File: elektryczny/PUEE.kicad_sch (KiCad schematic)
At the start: 61 parts, among them J1 CAN, J2 VIN, J4 Button1, J5 LED1, J6 Button2, J7 STM, J8 OLED, SW1 Button2, SW2 Button1, U1 STM32F042F4Px, U10 WS2815, U11 WS2815, U13 SN65HVD230QDRG4Q1, U2 ESP-12E, U3 TPS54308, U4 WS2815, U5 WS2815, U6 WS2815, U7 WS2815, U8 WS2815, U9 WS2815, Y2 ABL-8MHZ-B2

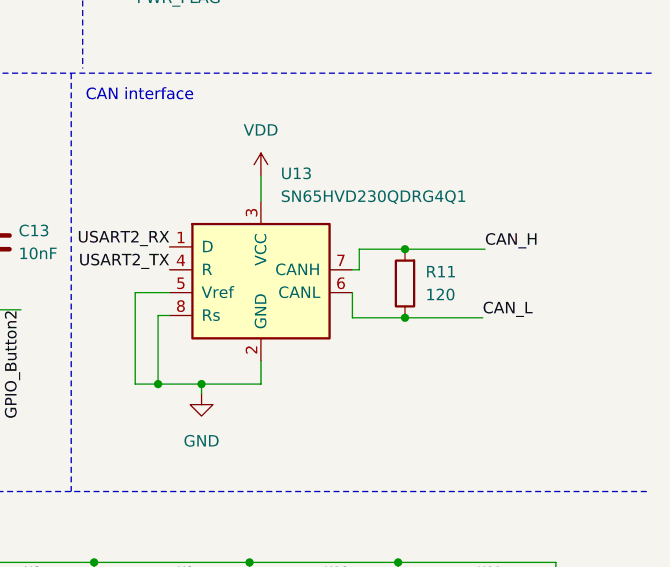
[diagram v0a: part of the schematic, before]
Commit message: polaczenia attempt 1, do poprawki
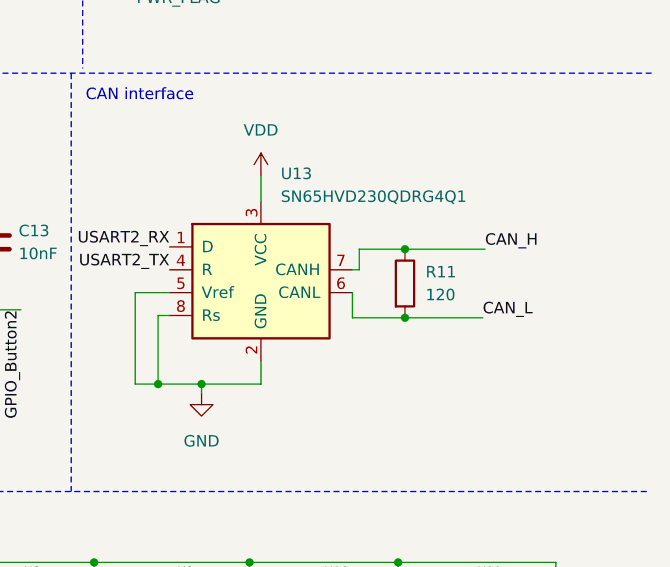
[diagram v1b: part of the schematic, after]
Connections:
- net CAN_H: now also R11.1; no longer R11.2
- net CAN_L: now also R11.2; no longer R11.1
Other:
- moved on the sheet: R11
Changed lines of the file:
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@@
 	)
 	(junction
-		(at 258.064 109.728)
+		(at 240.792 144.526)
 		(diameter 0)
 		(color 0 0 0 0)
 	)
 	(junction
-		(at 240.792 144.526)
+		(at 20.828 122.174)
 		(diameter 0)
 		(color 0 0 0 0)
 	)
 	(junction
-		(at 20.828 122.174)
+		(at 258.064 117.348)
 		(diameter 0)
 		(color 0 0 0 0)
@@
 	)
 	(junction
-		(at 258.064 117.348)
+		(at 258.064 109.728)
 		(diameter 0)
 		(color 0 0 0 0)
@@
 	(wire
 		(pts
-			(xy 258.064 117.348) (xy 266.7 117.348)
-		)
-		(stroke
-			(width 0)
-			(type default)
-		)
-	)
-	(wire
-		(pts
 			(xy 183.896 116.078) (xy 186.436 116.078)
 		)
@@
 	(wire
 		(pts
-			(xy 258.064 109.728) (xy 266.954 109.728)
+			(xy 206.756 162.052) (xy 206.756 163.322)
 		)
 		(stroke
@@
 	(wire
 		(pts
-			(xy 206.756 162.052) (xy 206.756 163.322)
+			(xy 201.422 126.111) (xy 201.422 127.508)
 		)
 		(stroke
@@
 	(wire
 		(pts
-			(xy 201.422 126.111) (xy 201.422 127.508)
+			(xy 75.692 65.278) (xy 81.28 65.278)
 		)
 		(stroke
@@
 	(wire
 		(pts
-			(xy 75.692 65.278) (xy 81.28 65.278)
+			(xy 251.714 28.702) (xy 251.714 39.116)
 		)
 		(stroke
@@
 	(wire
 		(pts
-			(xy 251.714 28.702) (xy 251.714 39.116)
+			(xy 171.45 116.078) (xy 173.482 116.078)
 		)
 		(stroke
@@
 	(wire
 		(pts
-			(xy 171.45 116.078) (xy 173.482 116.078)
+			(xy 16.51 52.324) (xy 18.034 52.324)
 		)
 		(stroke
@@
 	(wire
 		(pts
-			(xy 16.51 52.324) (xy 18.034 52.324)
+			(xy 173.482 104.902) (xy 173.482 105.41)
 		)
 		(stroke
@@
 	(wire
 		(pts
-			(xy 173.482 104.902) (xy 173.482 105.41)
+			(xy 258.064 109.728) (xy 266.954 109.728)
 		)
 		(stroke
@@
 	(wire
 		(pts
+			(xy 258.064 117.348) (xy 266.7 117.348)
+		)
+		(stroke
+			(width 0)
+			(type default)
+		)
+	)
+	(wire
+		(pts
 			(xy 176.276 116.078) (xy 173.482 116.078)
 		)
@@
 	(symbol
 		(lib_id "Device:R")
-		(at 258.064 113.538 180)
+		(at 258.064 113.538 0)
 		(unit 1)
 		(exclude_from_sim no)
@@
 					(size 1.27 1.27)
 				)
-				(justify right)
+				(justify left)
 			)
 		)
@@
 					(size 1.27 1.27)
 				)
-				(justify right)
+				(justify left)
 			)
 		)
 		(property "Footprint" "Resistor_SMD:R_0805_2012Metric"
-			(at 259.842 113.538 90)
+			(at 256.286 113.538 90)
 			(effects
 				(font
